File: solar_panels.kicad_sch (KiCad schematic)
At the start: 1 part, among them J1 Conn_01x04_Pin

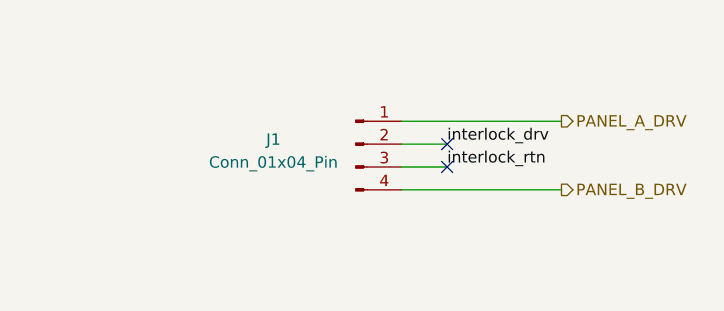
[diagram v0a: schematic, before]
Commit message: Cleaning up schematic
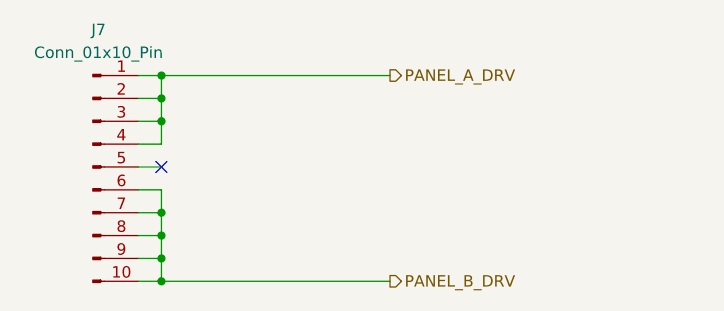
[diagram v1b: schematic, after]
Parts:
- removed J1: Conn_01x04_Pin, symbol Connector:Conn_01x04_Pin
- added J7: Conn_01x10_Pin, symbol Connector:Conn_01x10_Pin
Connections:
- net PANEL_A_DRV: now also J7.1 (Pin_1), J7.2 (Pin_2), J7.3 (Pin_3), J7.4 (Pin_4)
- net PANEL_B_DRV: now also J7.10 (Pin_10), J7.6 (Pin_6), J7.7 (Pin_7), J7.8 (Pin_8), J7.9 (Pin_9)
- no-connect marks 2 -> 1
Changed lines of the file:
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@@
 		(comment 3 "Reviewer 2:")
 	)
+	(junction
+		(at 106.68 107.95)
+		(diameter 0)
+		(color 0 0 0 0)
+	)
+	(junction
+		(at 106.68 95.25)
+		(diameter 0)
+		(color 0 0 0 0)
+	)
+	(junction
+		(at 106.68 113.03)
+		(diameter 0)
+		(color 0 0 0 0)
+	)
+	(junction
+		(at 106.68 105.41)
+		(diameter 0)
+		(color 0 0 0 0)
+	)
+	(junction
+		(at 106.68 90.17)
+		(diameter 0)
+		(color 0 0 0 0)
+	)
+	(junction
+		(at 106.68 92.71)
+		(diameter 0)
+		(color 0 0 0 0)
+	)
+	(junction
+		(at 106.68 110.49)
+		(diameter 0)
+		(color 0 0 0 0)
+	)
 	(no_connect
-		(at 138.43 97.79)
-	)
-	(no_connect
-		(at 138.43 100.33)
-	)
-	(wire
-		(pts
-			(xy 133.35 102.87) (xy 151.13 102.87)
-		)
-		(stroke
-			(width 0)
-			(type default)
-		)
-	)
-	(wire
-		(pts
-			(xy 133.35 95.25) (xy 151.13 95.25)
-		)
-		(stroke
-			(width 0)
-			(type default)
-		)
-	)
-	(wire
-		(pts
-			(xy 133.35 100.33) (xy 138.43 100.33)
-		)
-		(stroke
-			(width 0)
-			(type default)
-		)
-	)
-	(wire
-		(pts
-			(xy 133.35 97.79) (xy 138.43 97.79)
-		)
-		(stroke
-			(width 0)
-			(type default)
-		)
-	)
-	(label "interlock_drv"
-		(at 138.43 97.79 0)
+		(at 106.68 100.33)
+	)
+	(wire
+		(pts
+			(xy 104.14 97.79) (xy 106.68 97.79)
+		)
+		(stroke
+			(width 0)
+			(type default)
+		)
+	)
+	(wire
+		(pts
+			(xy 104.14 90.17) (xy 106.68 90.17)
+		)
+		(stroke
+			(width 0)
+			(type default)
+		)
+	)
+	(wire
+		(pts
+			(xy 106.68 110.49) (xy 106.68 107.95)
+		)
+		(stroke
+			(width 0)
+			(type default)
+		)
+	)
+	(wire
+		(pts
+			(xy 106.68 92.71) (xy 106.68 95.25)
+		)
+		(stroke
+			(width 0)
+			(type default)
+		)
+	)
+	(wire
+		(pts
+			(xy 106.68 113.03) (xy 132.08 113.03)
+		)
+		(stroke
+			(width 0)
+			(type default)
+		)
+	)
+	(wire
+		(pts
+			(xy 106.68 90.17) (xy 106.68 92.71)
+		)
+		(stroke
+			(width 0)
+			(type default)
+		)
+	)
+	(wire
+		(pts
+			(xy 106.68 90.17) (xy 132.08 90.17)
+		)
+		(stroke
+			(width 0)
+			(type default)
+		)
+	)
+	(wire
+		(pts
+			(xy 104.14 110.49) (xy 106.68 110.49)
+		)
+		(stroke
+			(width 0)
+			(type default)
+		)
+	)
+	(wire
+		(pts
+			(xy 106.68 95.25) (xy 106.68 97.79)
+		)
+		(stroke
+			(width 0)
+			(type default)
+		)
+	)
+	(wire
+		(pts
+			(xy 104.14 95.25) (xy 106.68 95.25)
+		)
+		(stroke
+			(width 0)
+			(type default)
+		)
+	)
+	(wire
+		(pts
+			(xy 104.14 105.41) (xy 106.68 105.41)
+		)
+		(stroke
+			(width 0)
+			(type default)
+		)
+	)
+	(wire
+		(pts
+			(xy 104.14 113.03) (xy 106.68 113.03)
+		)
+		(stroke
+			(width 0)
+			(type default)
+		)
+	)
+	(wire
+		(pts
+			(xy 106.68 113.03) (xy 106.68 110.49)
+		)
+		(stroke
+			(width 0)
+			(type default)
+		)
+	)
+	(wire
+		(pts
+			(xy 104.14 107.95) (xy 106.68 107.95)
+		)
+		(stroke
+			(width 0)
+			(type default)
+		)
+	)
+	(wire
+		(pts
+			(xy 104.14 92.71) (xy 106.68 92.71)
+		)
+		(stroke
+			(width 0)
+			(type default)
+		)
+	)
+	(wire
+		(pts
+			(xy 106.68 107.95) (xy 106.68 105.41)
+		)
+		(stroke
+			(width 0)
+			(type default)
+		)
+	)
+	(wire
+		(pts
+			(xy 104.14 102.87) (xy 106.68 102.87)
+		)
+		(stroke
+			(width 0)
+			(type default)
+		)
+	)
+	(wire
+		(pts
+			(xy 104.14 100.33) (xy 106.68 100.33)
+		)
+		(stroke
+			(width 0)
+			(type default)
+		)
+	)
+	(wire
+		(pts
+			(xy 106.68 105.41) (xy 106.68 102.87)
+		)
+		(stroke
+			(width 0)
+			(type default)
+		)
+	)
+	(hierarchical_label "PANEL_A_DRV"
+		(shape output)
+		(at 132.08 90.17 0)
 		(effects
 			(font
 				(size 1.27 1.27)
 			)
-			(justify left bottom)
-		)
-	)
-	(label "interlock_rtn"
-		(at 138.43 100.33 0)
+			(justify left)
+		)
+	)
+	(hierarchical_label "PANEL_B_DRV"
+		(shape output)
+		(at 132.08 113.03 0)
 		(effects
 			(font
 				(size 1.27 1.27)
 			)
-			(justify left bottom)
-		)
-	)
-	(hierarchical_label "PANEL_A_DRV"
-		(shape output)
-		(at 151.13 95.25 0)
-		(effects
-			(font
-				(size 1.27 1.27)
-			)
 			(justify left)
 		)
 	)
-	(hierarchical_label "PANEL_B_DRV"
-		(shape output)
-		(at 151.13 102.87 0)
-		(effects
-			(font
-				(size 1.27 1.27)
-			)
-			(justify left)
-		)
-	)
 	(symbol
-		(lib_id "Connector:Conn_01x04_Pin")
-		(at 128.27 97.79 0)
+		(lib_id "Connector:Conn_01x10_Pin")
+		(at 99.06 100.33 0)
 		(unit 1)
 		(exclude_from_sim no)
@@
 		(on_board yes)
 		(dnp no)
-		(property "Reference" "J1"
-			(at 119.126 97.282 0)
-			(effects
-				(font
-					(size 1.27 1.27)
-				)
-			)
-		)
-		(property "Value" "Conn_01x04_Pin"
-			(at 119.126 99.822 0)
+		(fields_autoplaced yes)
+		(property "Reference" "J7"
+			(at 99.695 85.09 0)
+			(effects
+				(font
+					(size 1.27 1.27)
+				)
+			)
+		)
+		(property "Value" "Conn_01x10_Pin"
+			(at 99.695 87.63 0)
 			(effects
 				(font
@@
 		)
 		(property "Footprint" ""
-			(at 128.27 97.79 0)
+			(at 99.06 100.33 0)
 			(effects
 				(font
@@
 		)
 		(property "Datasheet" "~"
-			(at 128.27 97.79 0)
+			(at 99.06 100.33 0)
 			(effects
 				(font
@@
 			)
 		)
-		(property "Description" "Generic connector, single row, 01x04, script generated"
-			(at 128.27 97.79 0)
+		(property "Description" "Generic connector, single row, 01x10, script generated"
+			(at 99.06 100.33 0)
 			(effects
 				(font
@@
 			)
 		)
+		(pin "9"
+		)
+		(pin "10"
+		)
 		(pin "2"
 		)
 		(pin "1"
 		)
+		(pin "3"
+		)
+		(pin "6"
+		)
 		(pin "4"
 		)
-		(pin "3"
+		(pin "8"
+		)
+		(pin "7"
+		)
+		(pin "5"
 		)
 		(instances
 			(project ""
 				(path "/99785679-20de-4827-b4cc-bc3c187068c9/9564929a-642e-4163-88c2-45054b63a5ed/84e96f9f-2d05-4b14-bccc-57bd87440548"
-					(reference "J1")
+					(reference "J7")
 					(unit 1)
 				)
